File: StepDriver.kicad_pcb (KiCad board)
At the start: 2 copper layers, 43.2 x 43.2 mm, 50 parts, among them IC1 MCP25625-E_ML, J1 SW, J2 Conn_01x05, J3 SERIAL, J4 ICSP, J5 I2C, J7 Terminals_01x04, J8 ENCODER, Q1 SI3415A, U1 ATMEGA328P-AU, U2 uA7805, Y1 OSCILLATOR-16MHZ, Y2 OSCILLATOR-16MHZ

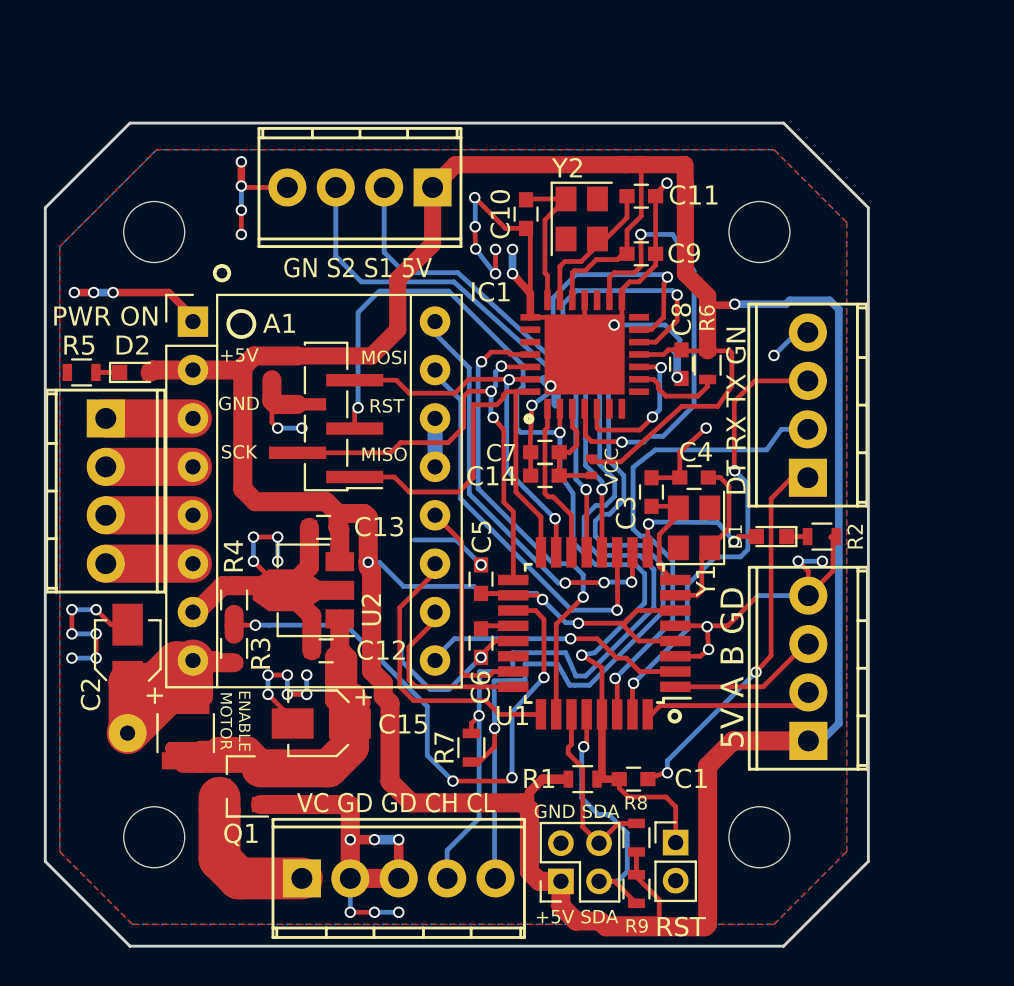
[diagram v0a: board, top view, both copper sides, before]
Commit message: Small changes, added step and refined schematic and images
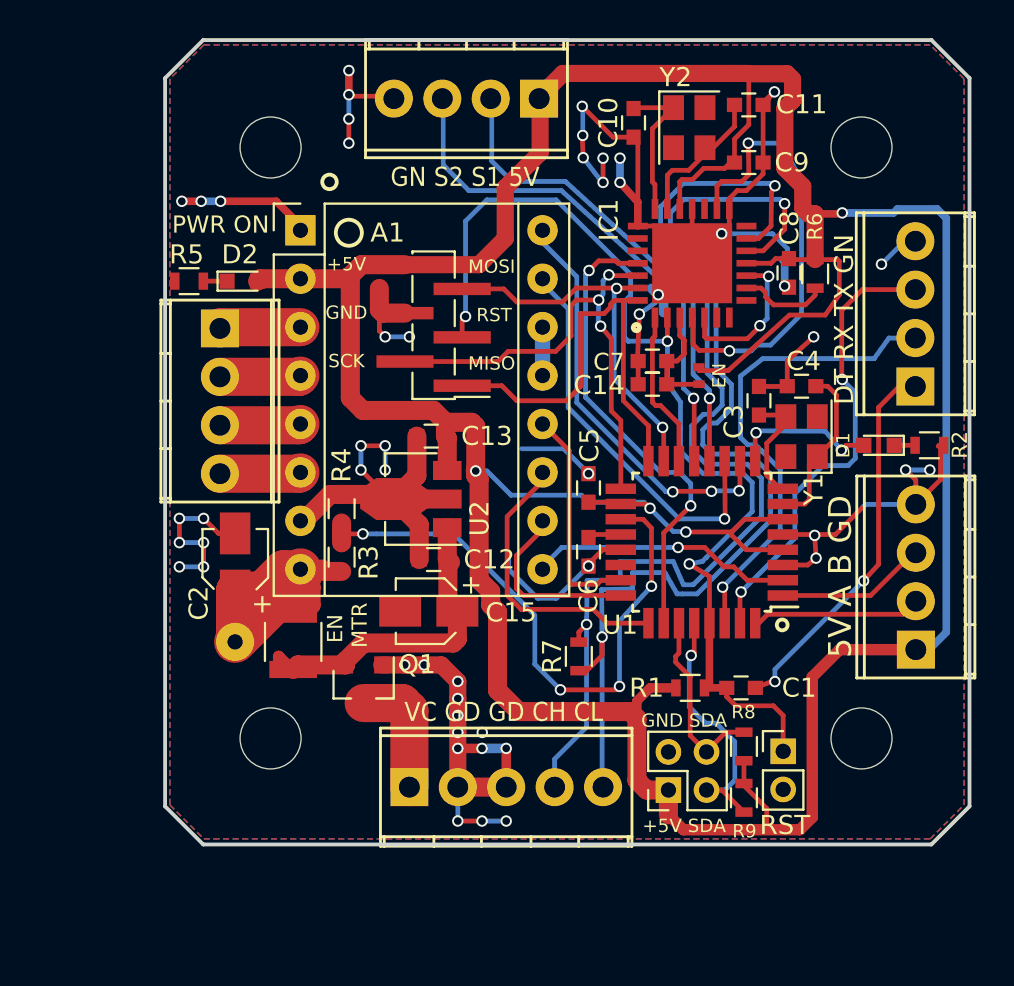
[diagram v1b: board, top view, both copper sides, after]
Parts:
- moved Q1 8.37 mm to (136.6, 111.2), turned to 270 degrees
- moved C15 8.15 mm to (140.0, 107.4)
- moved J7 7.63 mm to (129.1, 92.6)
- moved MK1 7.40 mm to (131.2, 82.7)
- moved MK4 7.40 mm to (131.2, 114.5)
- moved C11 7.40 mm to (156.8, 80.8)
- moved C12 7.40 mm to (140.3, 104.7)
- moved C14 7.40 mm to (151.7, 95.5)
- moved C7 7.40 mm to (151.7, 94.3)
- moved C8 7.40 mm to (158.9, 89.6)
- moved C9 7.40 mm to (156.8, 83.9)
- moved D1 7.40 mm to (163.6, 98.7)
- moved J2 7.40 mm to (139.0, 116.6)
- moved J3 7.40 mm to (165.5, 95.6)
- moved J4 7.40 mm to (140.3, 92.4)
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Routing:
- net VCC: track 32.1 -> 18.1 mm
- net GND: track 169.6 -> 163.8 mm, vias 51 -> 52
- net INPUT_VCC: track 9.29 -> 6.59 mm
- net +5V: track 212.8 -> 211.3 mm
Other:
- board size 43.2 x 43.2 mm -> 42.2 x 42.2 mm
- board text added: "EN"
- board text added: "EN MTR"
- board text removed: "ENABLE MOTOR"
- board text removed: "VCC"
